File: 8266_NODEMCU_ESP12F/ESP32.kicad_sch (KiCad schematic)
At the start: 6 parts, among them J1 Screw_Terminal_01x02, J2 Screw_Terminal_01x02, Q1 IRLZ44N, U1 NodeMCU_ESP8266_LUA_12-F, U2 Generic_5v_Module

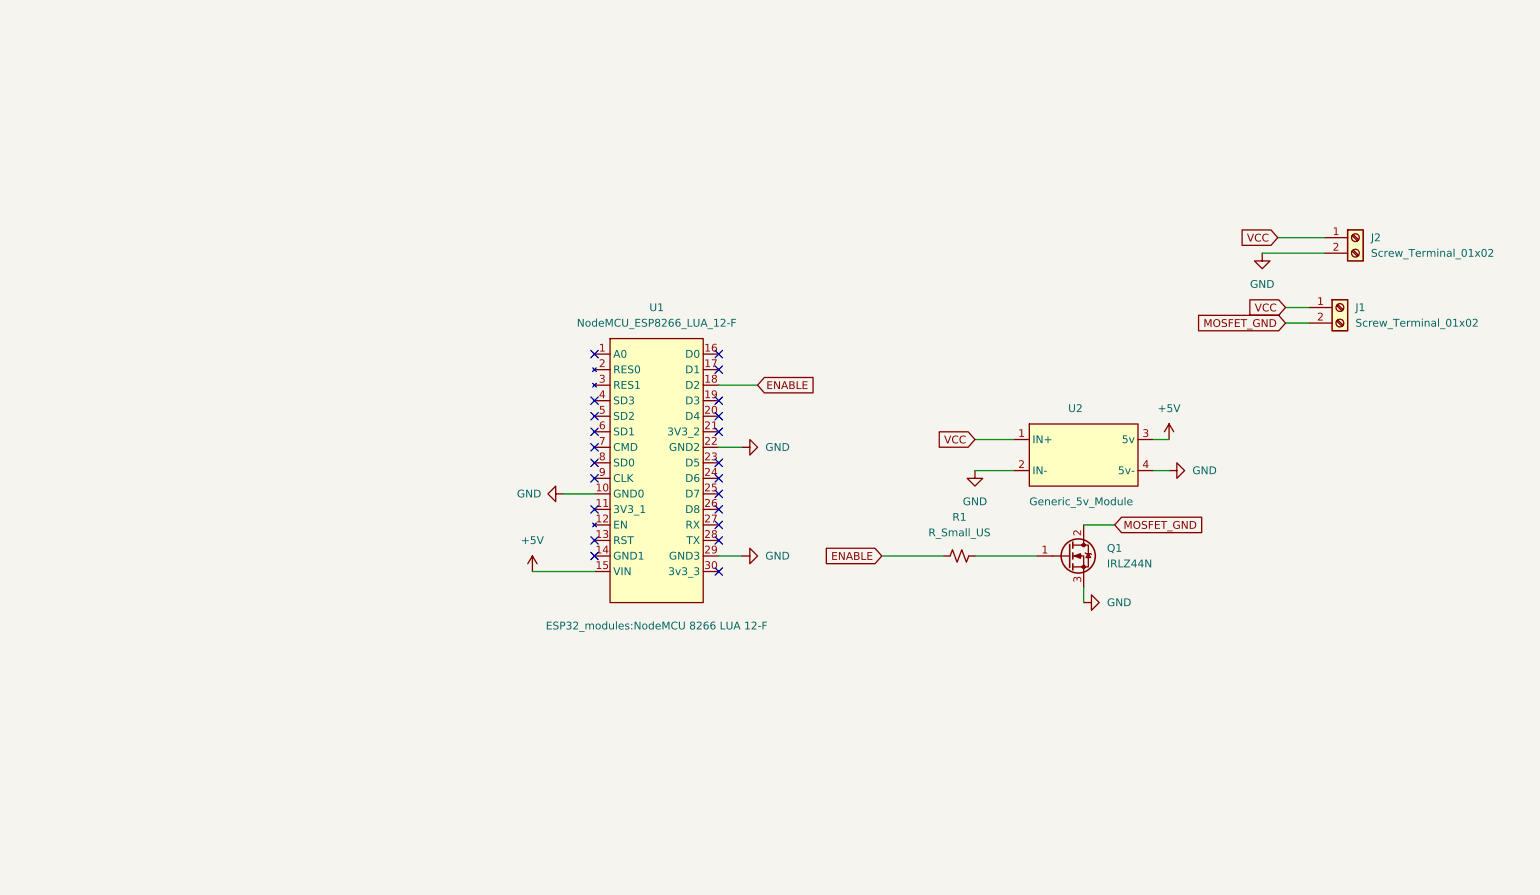
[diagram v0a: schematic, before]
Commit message: KiCad Updates
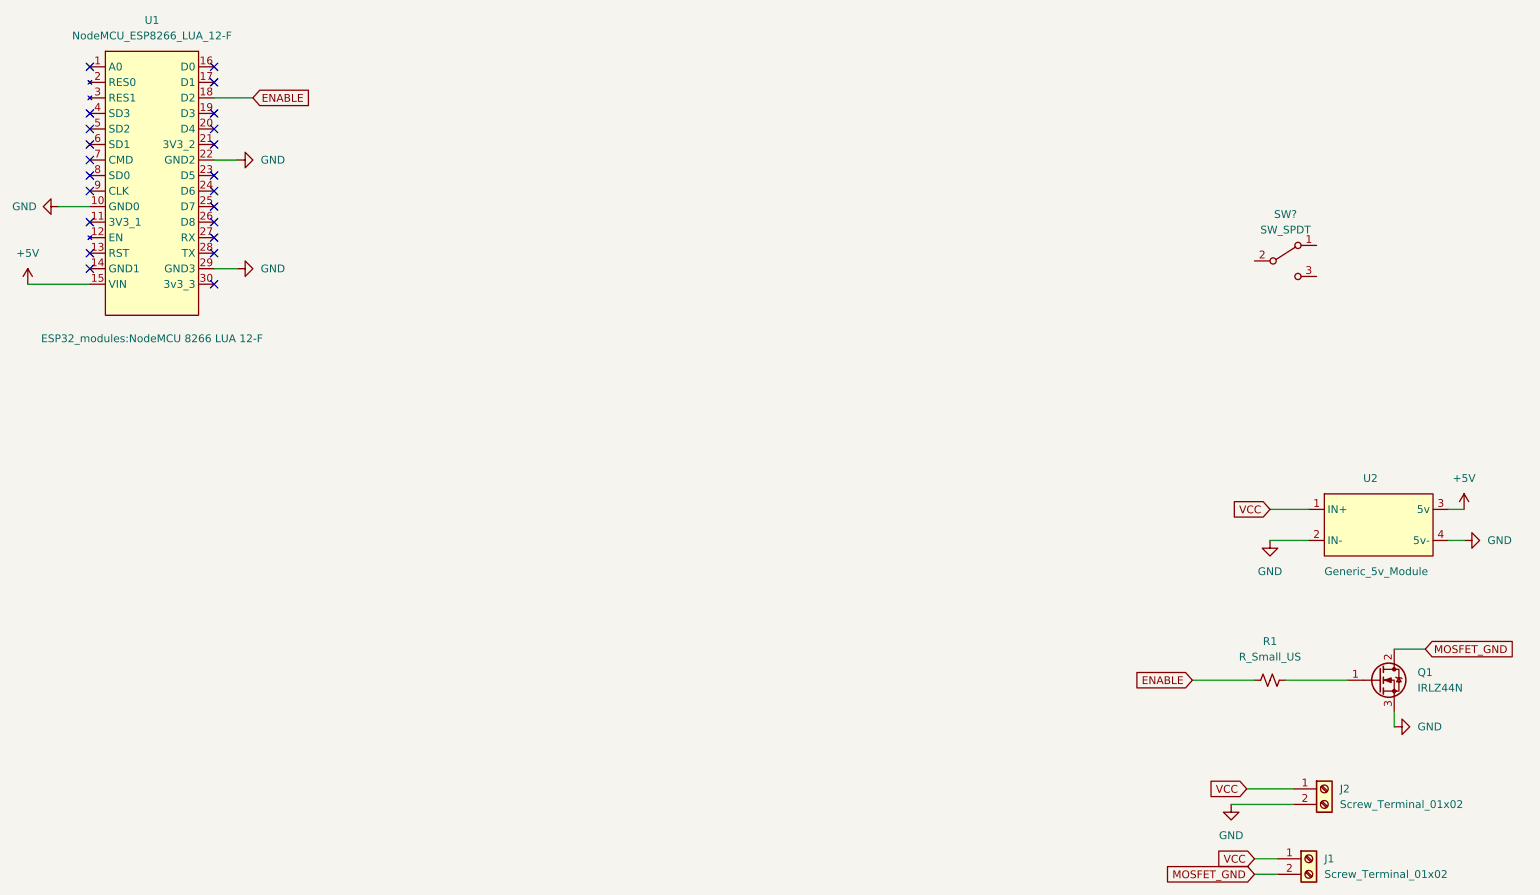
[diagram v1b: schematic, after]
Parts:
- added SW?: SW_SPDT, symbol Switch:SW_SPDT
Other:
- moved on the sheet: J1, J2, Q1, R1, U1, U2
